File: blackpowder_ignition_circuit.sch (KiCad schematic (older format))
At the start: 12 parts, among them J2 Conn_01x02, J3 Conn_01x02, Q1 FDS6898A, Q2 FDS6898A, U2 TC4427AVOA

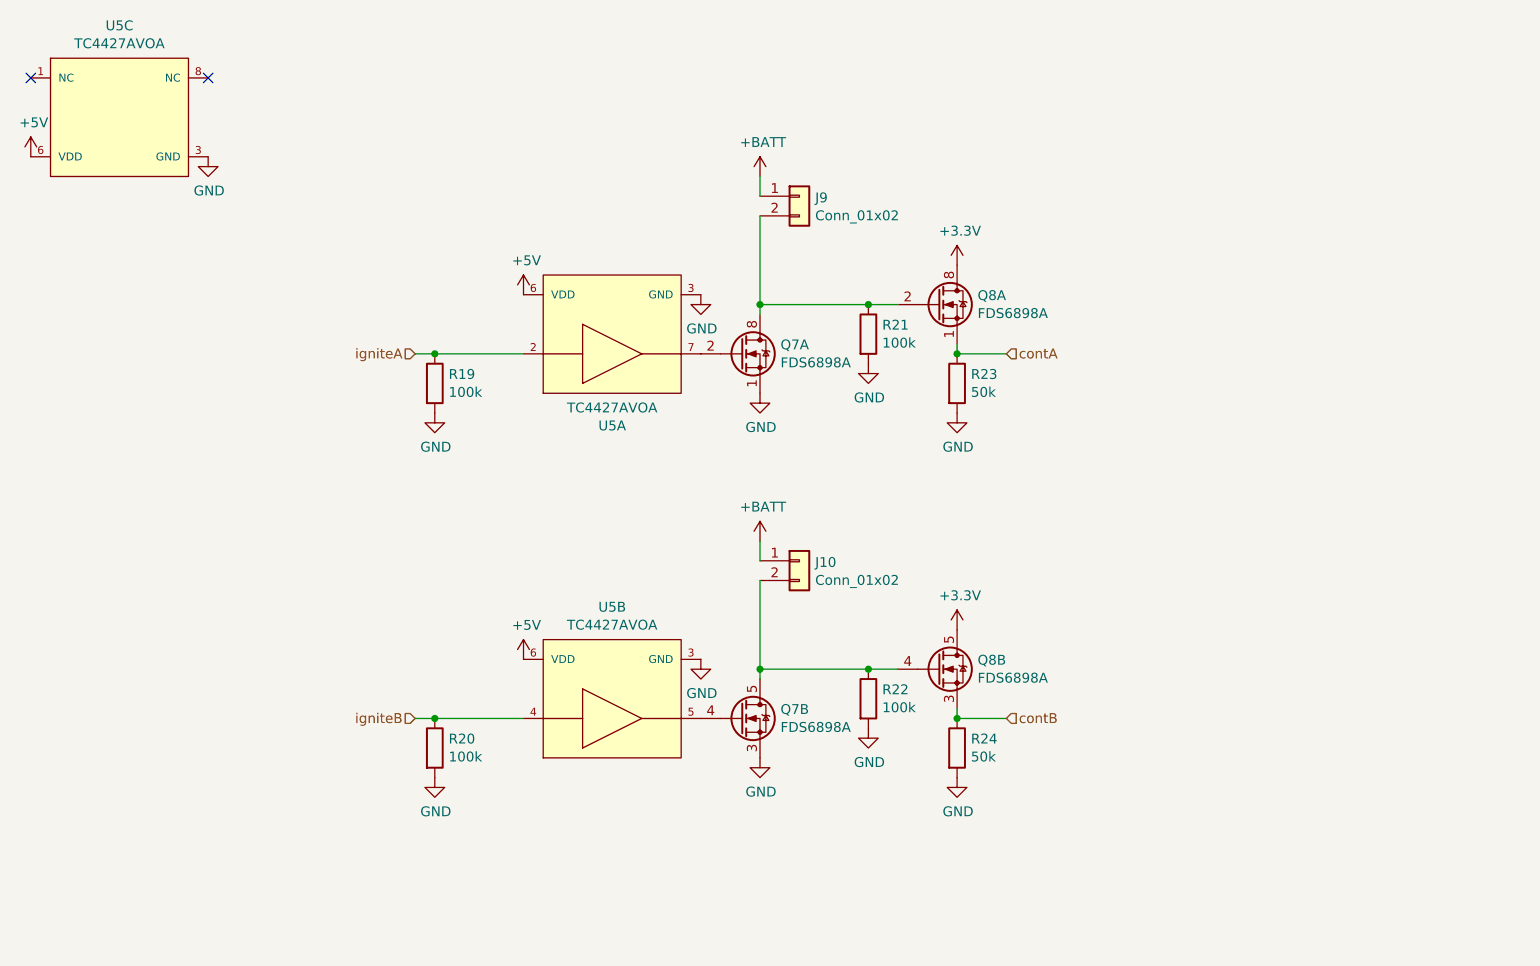
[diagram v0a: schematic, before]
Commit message: addressed review comments
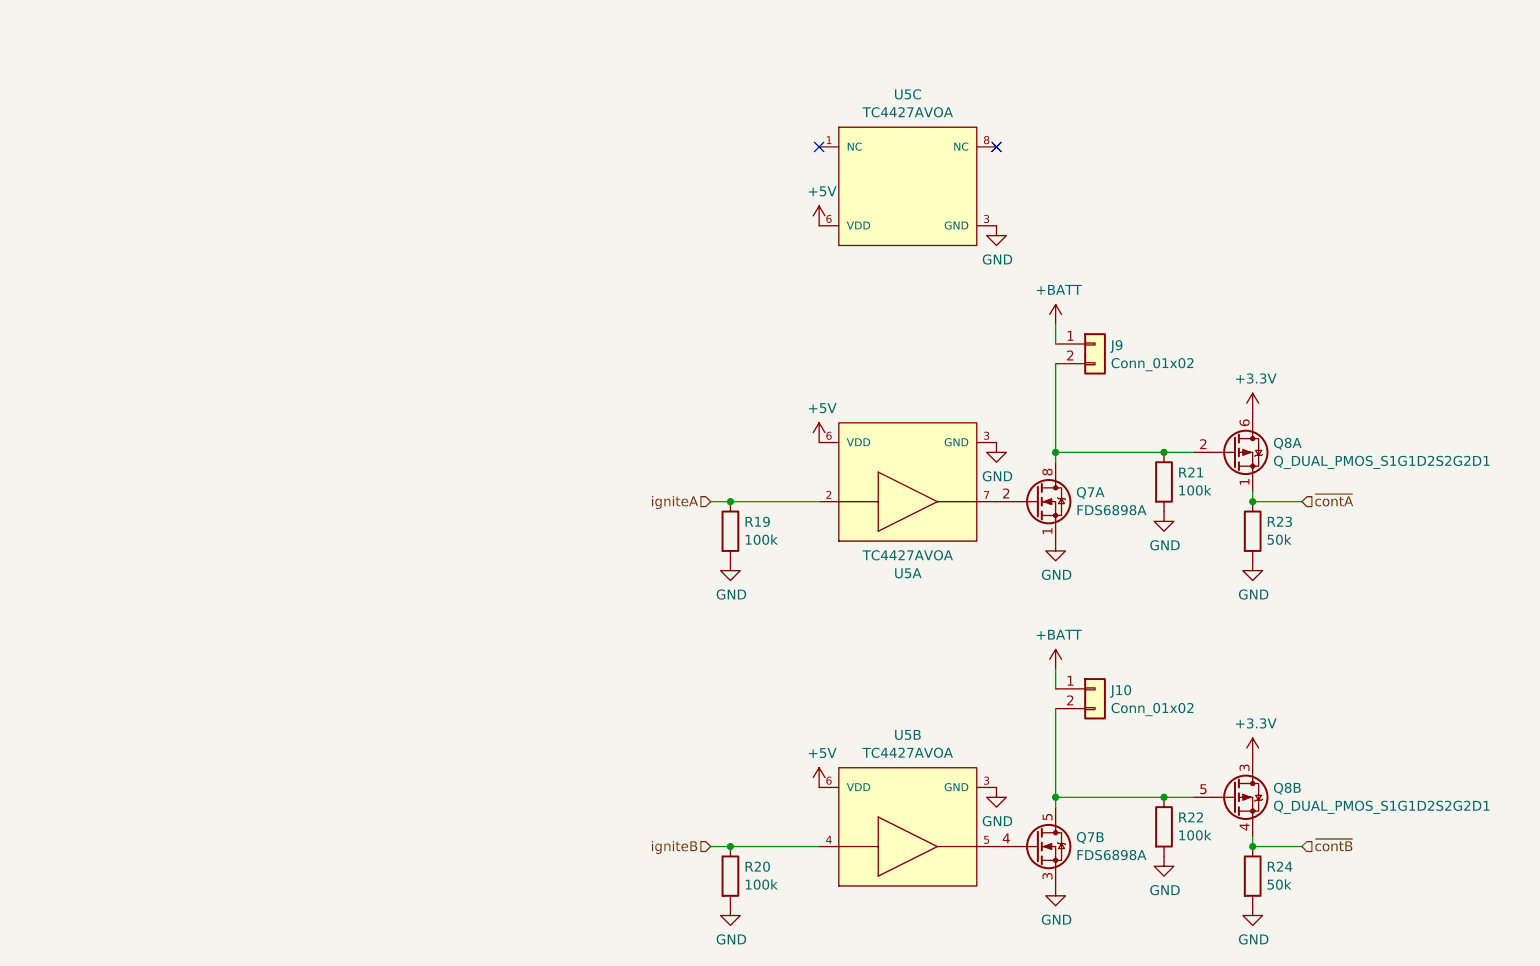
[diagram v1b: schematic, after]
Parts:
- removed Q1, Q2: FDS6898A, Package_SO:SOIC-8_3.9x4.9mm_P1.27mm, symbol Transistor_FET:FDS6898A
- added Q2: Q_DUAL_PMOS_S1G1D2S2G2D1, Package_TO_SOT_SMD:SOT-363_SC-70-6_Handsoldering, symbol Device:Q_DUAL_PMOS_S1G1D2S2G2D1
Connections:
- net +3V3: now also Q2.3 (D), Q2.6 (D)
- net at J2.2 (Pin_2), Q1.7 (D1), Q1.8 (D1)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: now also Q2.2 (G)
- net at J3.2 (Pin_2), Q1.5 (D2), Q1.6 (D2)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: now also Q2.5 (G)
- net contA renamed ~contA~
- net ~contA~: now also Q2.1 (S)
- net contB renamed ~contB~
- net ~contB~: now also Q2.4 (S)
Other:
- moved on the sheet: J10, J9, Q7A, Q7B, R19, R20, R21, R22, R23, R24, U5A, U5B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
